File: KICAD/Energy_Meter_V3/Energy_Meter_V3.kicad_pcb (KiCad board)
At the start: 2 copper layers, 125 parts, among them J1 Conn_01x04_Socket, J2 Conn_01x02_Pin, J3 Conn_01x02_Pin, J4 Conn_01x02_Pin, J5 Conn_01x04_Socket, J6 Conn_01x04_Socket, J7 Barrel_Jack_Switch_Pin3Ring, J8 USB_C_Receptacle_USB2.0_16P, J9 USB_C_Receptacle_USB2.0_16P, Q1 Q_NPN_BEC, U1 ADE7758, U3 STM32F103C8Tx, U4 XL1509-5.0, U5 AMS1117-5.0, U6 ESP32-C3-WROOM-02U, Y1 10M, Y2 32.768k, Y3 8M, Y4 32.768k

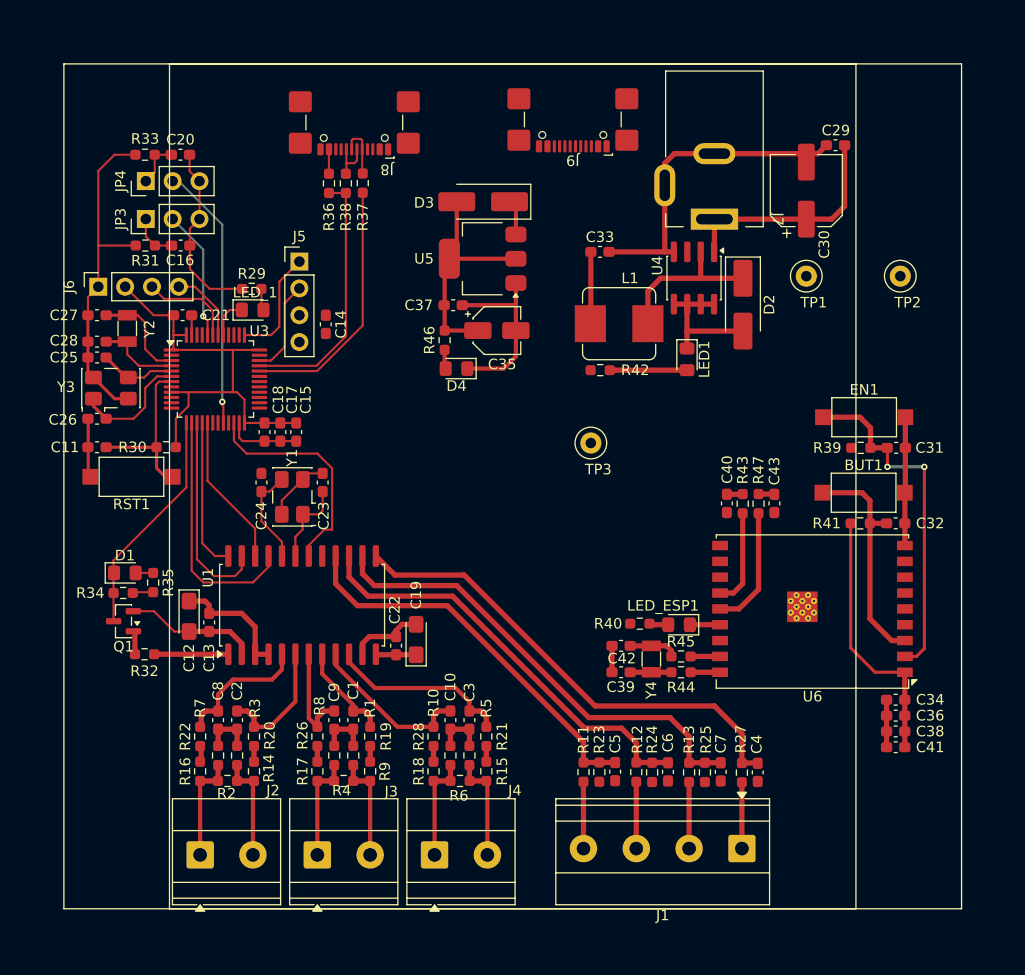
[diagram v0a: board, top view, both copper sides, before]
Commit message: upload 80%
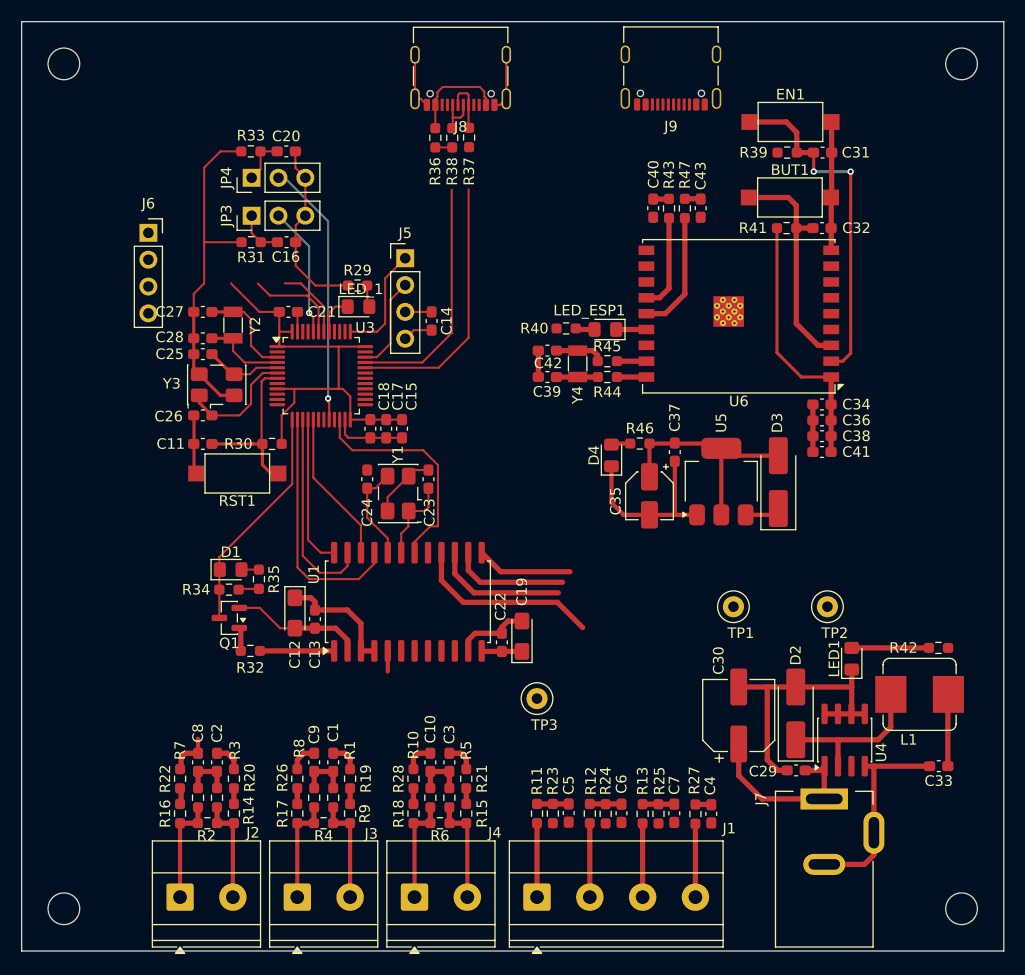
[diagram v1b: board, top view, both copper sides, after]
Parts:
- J8, J9: footprint Connector_USB:USB_C_Receptacle_GCT_USB4110 -> Connector_USB:USB_C_Receptacle_Palconn_UTC16-G
- moved C29 59.3 mm to (149.6, 103.7)
- moved C33 58.3 mm to (163.1, 103.3), turned to 0 degrees
- moved J7 55.9 mm to (152.3, 106.4), turned to 90 degrees
- moved C30 50.1 mm to (144.2, 98.5)
- moved U4 46.0 mm to (154.2, 100.8), turned to 90 degrees
- moved L1 45.2 mm to (161.3, 96.5), turned to 0 degrees
- moved R42 41.4 mm to (163.1, 92.1), turned to 180 degrees
- moved D2 39.0 mm to (149.6, 98.3), turned to 90 degrees
- moved D3 38.6 mm to (147.9, 76.4), turned to 90 degrees
- moved LED1 32.4 mm to (154.9, 93.1), turned to 90 degrees
- moved TP1 32.1 mm to (143.7, 88.2)
- moved TP2 32.1 mm to (152.6, 88.2)
- moved U5 30.9 mm to (142.6, 76.3), turned to 90 degrees
- moved R40 28.8 mm to (127.9, 61.9)
- moved C31 28.8 mm to (152.1, 45.2)
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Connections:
- J1 pad 1: /N -> /A
- J1 pad 2: /C -> /B
- J1 pad 3: /B -> /C
- J1 pad 4: /A -> /N
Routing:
- net /VN: track 45.9 -> 10.9 mm
- net /VCP: track 44.5 -> 14.2 mm
- net /VBP: track 40.6 -> 15.7 mm
- net /VAP: track 37.3 -> 20.8 mm
- net /ICN: track 17.4 -> 2.79 mm
- net GND1: track 123.5 -> 137.1 mm
- net /ICP: track 15.6 -> 2.85 mm
- net /IAN: track 12.1 -> 2.73 mm
- net +5V: track 24.1 -> 31.5 mm
- net /IBP: track 9.94 -> 2.73 mm
- net /IAP: track 12.9 -> 6.18 mm
- net /IBN: track 9.39 -> 2.79 mm
- net +12V: track 21.7 -> 17.1 mm
- net GNDPWR: track 43.9 -> 47.5 mm
- net 3.3V: track 109.0 -> 111.9 mm
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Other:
- board outline added: 93 x 88 mm
